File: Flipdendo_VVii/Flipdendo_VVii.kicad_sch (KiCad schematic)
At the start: 0 parts

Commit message: librad ja asjalibrad ja asjadd
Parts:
- added IC1: TPS54429PWPR, SOP65P640X120-15N, symbol TPS54429PWPR:TPS54429PWPR
- added J1: Barrel_Jack, symbol Connector:Barrel_Jack
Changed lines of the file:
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@@
 	(generator_version "9.0")
 	(paper "A4")
+	(symbol
+		(lib_id "TPS54429PWPR:TPS54429PWPR")
+		(at 68.58 36.83 0)
+		(unit 1)
+		(exclude_from_sim no)
+		(in_bom yes)
+		(on_board yes)
+		(dnp no)
+		(fields_autoplaced yes)
+		(property "Reference" "IC1"
+			(at 83.82 29.21 0)
+			(effects
+				(font
+					(size 1.27 1.27)
+				)
+			)
+		)
+		(property "Value" "TPS54429PWPR"
+			(at 83.82 31.75 0)
+			(effects
+				(font
+					(size 1.27 1.27)
+				)
+			)
+		)
+		(property "Footprint" "SOP65P640X120-15N"
+			(at 95.25 131.75 0)
+			(effects
+				(font
+					(size 1.27 1.27)
+				)
+				(justify left top)
+				(hide yes)
+			)
+		)
+		(property "Datasheet" "http://www.ti.com/lit/gpn/tps54429"
+			(at 95.25 231.75 0)
+			(effects
+				(font
+					(size 1.27 1.27)
+				)
+				(justify left top)
+				(hide yes)
+			)
+		)
+		(property "Description" "7V to 18V Input, 4.5A Synchronous Step-Down DCAP2 Mode Converter"
+			(at 84.074 26.162 0)
+			(effects
+				(font
+					(size 1.27 1.27)
+				)
+				(hide yes)
+			)
+		)
+		(property "Height" "1.2"
+			(at 95.25 431.75 0)
+			(effects
+				(font
+					(size 1.27 1.27)
+				)
+				(justify left top)
+				(hide yes)
+			)
+		)
+		(property "Mouser Part Number" "595-TPS54429PWPR"
+			(at 95.25 531.75 0)
+			(effects
+				(font
+					(size 1.27 1.27)
+				)
+				(justify left top)
+				(hide yes)
+			)
+		)
+		(property "Mouser Price/Stock" "https://www.mouser.co.uk/ProductDetail/Texas-Instruments/TPS54429PWPR?qs=QtI0yD1FyONGxDVqigl07Q%3D%3D"
+			(at 95.25 631.75 0)
+			(effects
+				(font
+					(size 1.27 1.27)
+				)
+				(justify left top)
+				(hide yes)
+			)
+		)
+		(property "Manufacturer_Name" "Texas Instruments"
+			(at 95.25 731.75 0)
+			(effects
+				(font
+					(size 1.27 1.27)
+				)
+				(justify left top)
+				(hide yes)
+			)
+		)
+		(property "Manufacturer_Part_Number" "TPS54429PWPR"
+			(at 95.25 831.75 0)
+			(effects
+				(font
+					(size 1.27 1.27)
+				)
+				(justify left top)
+				(hide yes)
+			)
+		)
+		(pin "8"
+		)
+		(pin "9"
+		)
+		(pin "13"
+		)
+		(pin "10"
+		)
+		(pin "15"
+		)
+		(pin "12"
+		)
+		(pin "1"
+		)
+		(pin "4"
+		)
+		(pin "5"
+		)
+		(pin "11"
+		)
+		(pin "2"
+		)
+		(pin "14"
+		)
+		(pin "3"
+		)
+		(pin "6"
+		)
+		(pin "7"
+		)
+		(instances
+			(project ""
+				(path "/489224c0-ace1-4530-aa61-a5d03adf1434"
+					(reference "IC1")
+					(unit 1)
+				)
+			)
+		)
+	)
+	(symbol
+		(lib_id "Connector:Barrel_Jack")
+		(at 40.64 43.18 0)
+		(unit 1)
+		(exclude_from_sim no)
+		(in_bom yes)
+		(on_board yes)
+		(dnp no)
+		(fields_autoplaced yes)
+		(property "Reference" "J1"
+			(at 40.64 34.29 0)
+			(effects
+				(font
+					(size 1.27 1.27)
+				)
+			)
+		)
+		(property "Value" "Barrel_Jack"
+			(at 40.64 36.83 0)
+			(effects
+				(font
+					(size 1.27 1.27)
+				)
+			)
+		)
+		(property "Footprint" ""
+			(at 41.91 44.196 0)
+			(effects
+				(font
+					(size 1.27 1.27)
+				)
+				(hide yes)
+			)
+		)
+		(property "Datasheet" "~"
+			(at 41.91 44.196 0)
+			(effects
+				(font
+					(size 1.27 1.27)
+				)
+				(hide yes)
+			)
+		)
+		(property "Description" "DC Barrel Jack"
+			(at 40.64 43.18 0)
+			(effects
+				(font
+					(size 1.27 1.27)
+				)
+				(hide yes)
+			)
+		)
+		(pin "1"
+		)
+		(pin "2"
+		)
+		(instances
+			(project ""
+				(path "/489224c0-ace1-4530-aa61-a5d03adf1434"
+					(reference "J1")
+					(unit 1)
+				)
+			)
+		)
+	)
 	(sheet_instances
 		(path "/"

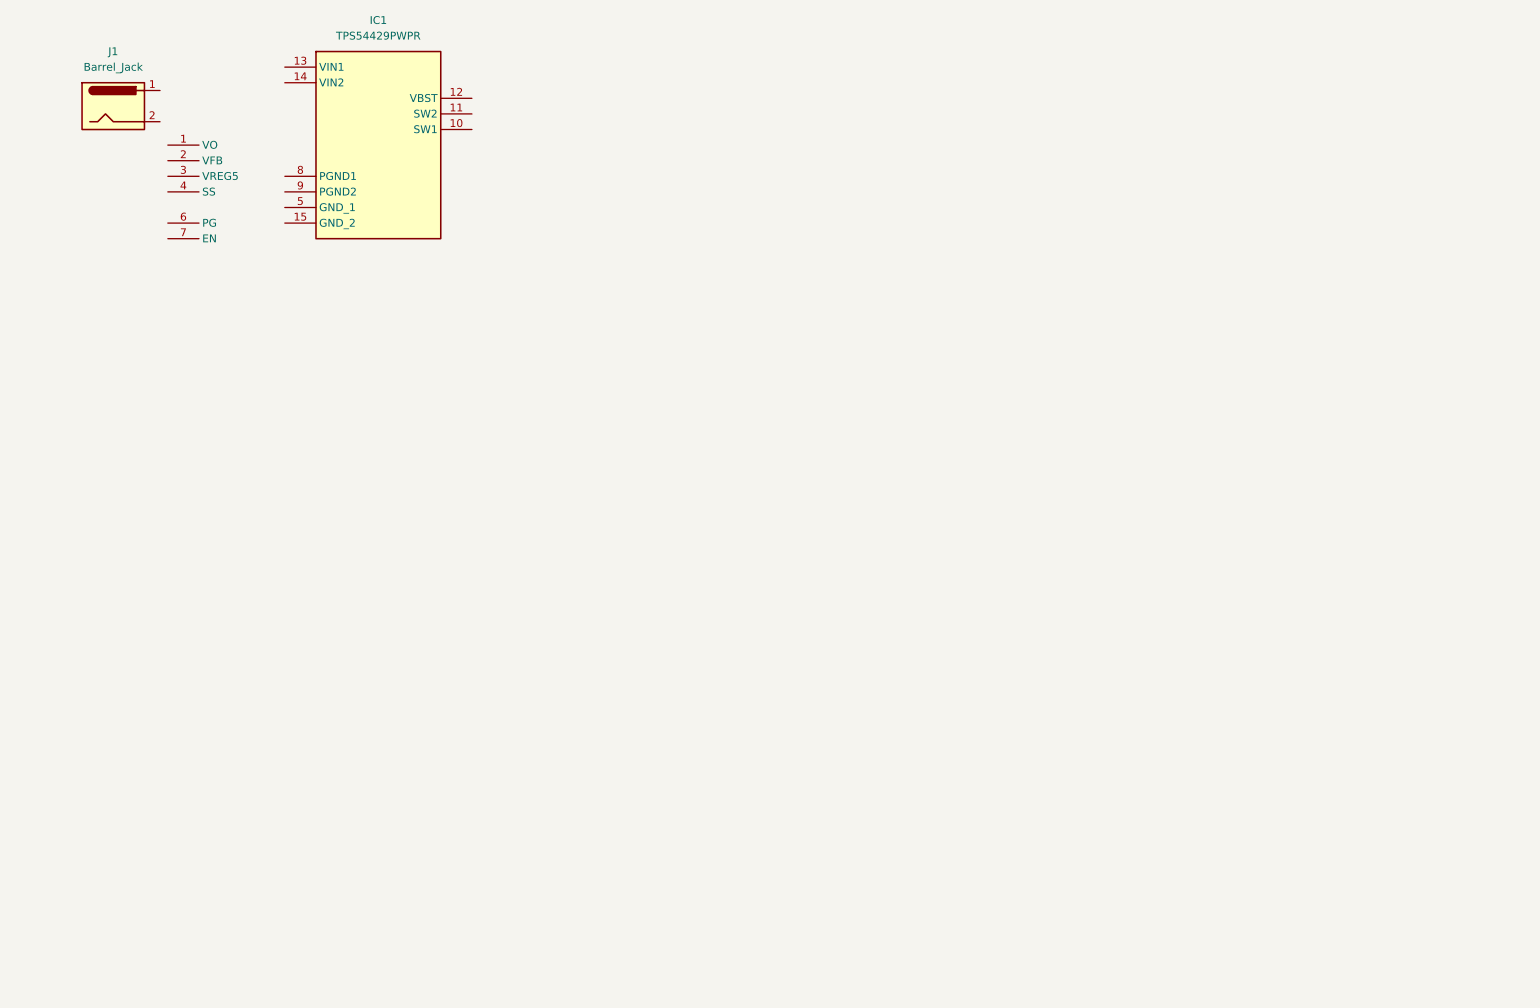
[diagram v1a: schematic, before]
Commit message: qwertytrerthgtrew
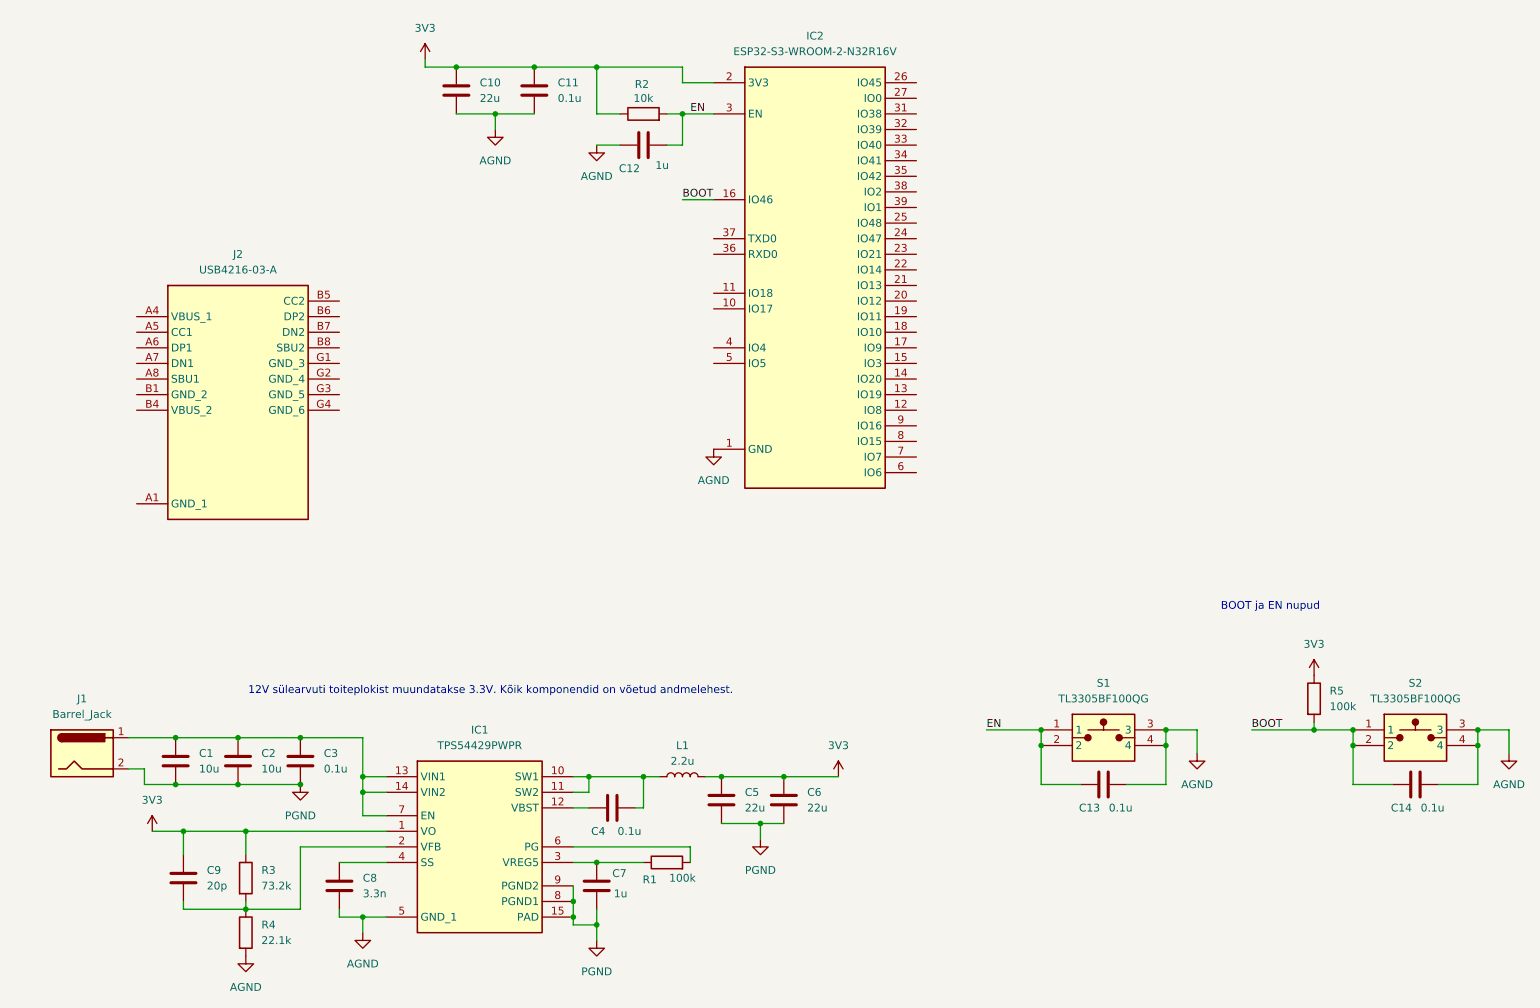
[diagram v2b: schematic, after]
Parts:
- added C1, C2: 10u, symbol Device:C
- added C10, C5, C6: 22u, symbol Device:C
- added C11, C13, C14, C3, C4: 0.1u, symbol Device:C
- added C12, C7: 1u, symbol Device:C
- added C8: 3.3n, symbol Device:C
- added C9: 20p, symbol Device:C
- added IC2: ESP32-S3-WROOM-2-N32R16V, ESP32S3WROOM2N32R16V, symbol ESP32-S3-WROOM-2-N32R16V:ESP32-S3-WROOM-2-N32R16V
- added J2: USB4216-03-A, USB421603A, symbol USB4216-03-A:USB4216-03-A
- added L1: 2.2u, symbol Device:L
- added R1, R5: 100k, symbol Device:R
- added R2: 10k, symbol Device:R
- added R3: 73.2k, symbol Device:R
- added R4: 22.1k, symbol Device:R
- added S1, S2: TL3305BF100QG, TL3305BF160QG, symbol TL3305BF100QG:TL3305BF100QG
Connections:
- net 3V3: now reaches IC1.1 (VO)
- net 3V3: now also C10.1, C11.1, C5.1, C6.1, C9.1, IC2.2 (3V3), L1.2, R2.1, R3.1, R5.1
- net at IC1.10 (SW1): now also IC1.11 (SW2), C4.2, L1.1
- net at IC1.12 (VBST): now also C4.1
- net at IC1.13 (VIN1): now also IC1.14 (VIN2), IC1.7 (EN), J1.1, C1.1, C2.1, C3.1
- net PGND: now reaches IC1.15 (PAD)
- net PGND: now also IC1.8 (PGND1), IC1.9 (PGND2), J1.2, C1.2, C2.2, C3.2, C5.2, C6.2, C7.2
- net at IC1.2 (VFB): now also C9.2, R3.2, R4.1
- net at IC1.3 (VREG5): now also C7.1, R1.1
- net at IC1.4 (SS): now also C8.1
- net AGND: now reaches IC1.5 (GND_1)
- net AGND: now also C10.2, C11.2, C12.1, C13.2, C14.2, C8.2, IC2.1 (GND), IC2.40 (GND), IC2.41 (GND), IC2.42 (GND), IC2.43 (GND), IC2.44 (GND), IC2.45 (GND), IC2.46 (GND), IC2.47 (GND), IC2.48 (GND), IC2.49 (GND), R4.2, S1.3, S1.4, S2.3, S2.4
- net at IC1.6 (PG): now also R1.2
- new net: IC2.28 (NC_1), IC2.29 (NC_2), IC2.30 (NC_3)
- new net BOOT: C14.1, IC2.16 (IO46), R5.2, S2.1, S2.2
- new net EN: C12.2, C13.1, IC2.3 (EN), R2.2, S1.1, S1.2
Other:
- note added: "12V sülearvuti toiteplokist muundatakse 3.3V. Kõik komponendid on võetud andmelehest."
- note added: "BOOT ja EN nupud"
- moved on the sheet: IC1, J1

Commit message: qwertyuiiiiuytrewwwertyuiuytrewertyuytrew
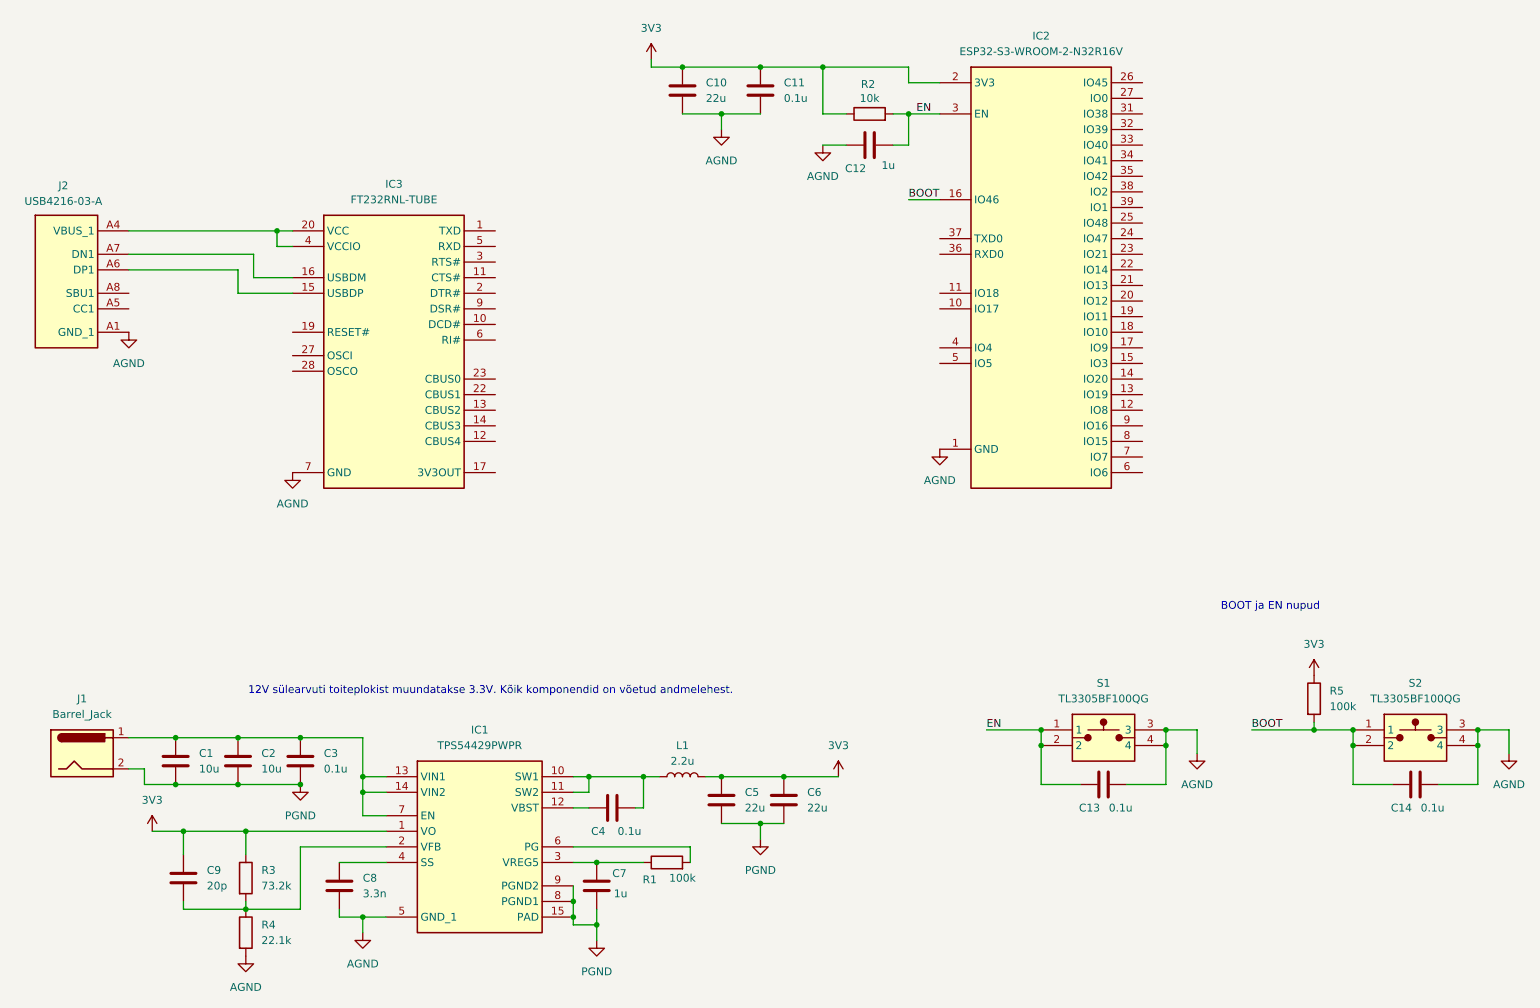
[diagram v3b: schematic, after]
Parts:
- added IC3: FT232RNL-TUBE, SOP65P780X200-28N, symbol FT232RNL-TUBE:FT232RNL-TUBE
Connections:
- net AGND: now also J2.A1 (GND_1), J2.B1 (GND_2), J2.G1 (GND_3), J2.G2 (GND_4), J2.G3 (GND_5), J2.G4 (GND_6), IC3.18 (GND_2), IC3.21 (GND_3), IC3.25 (AGND), IC3.7 (GND)
- net at J2.A4 (VBUS_1): now also J2.B4 (VBUS_2), IC3.20 (VCC), IC3.4 (VCCIO)
- net at J2.A5 (CC1): now also J2.B5 (CC2)
- net at J2.A6 (DP1): now also J2.B6 (DP2), IC3.15 (USBDP)
- net at J2.A7 (DN1): now also J2.B7 (DN2), IC3.16 (USBDM)
- net at J2.A8 (SBU1): now also J2.B8 (SBU2)
- new net: IC3.24 (NC_2), IC3.8 (NC_1)
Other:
- moved on the sheet: C10, C11, C12, IC2, R2
